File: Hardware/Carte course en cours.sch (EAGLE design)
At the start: 39 parts, among them J2 AVR_SPI_PROG_3X2NS, J3 PWR IN, J4 RC receiver, J5 ESC, J6 ESC, J7 MICRO-SD_CARD_SOCKET, J8 ESC, U1 V_REG_317SMD, U2 ATMEGA328P_TQFP, U3 FT232RL, U4 MPU6050, Y1 16MHz

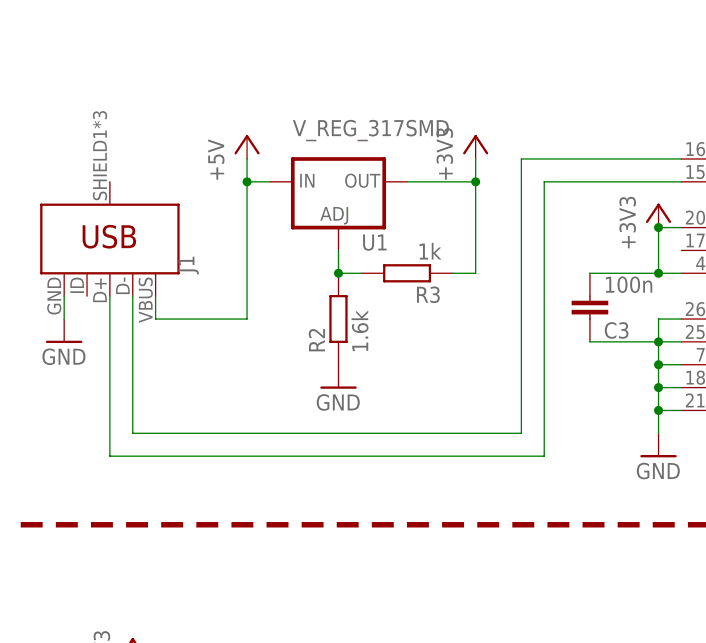
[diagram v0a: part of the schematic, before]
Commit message: Route
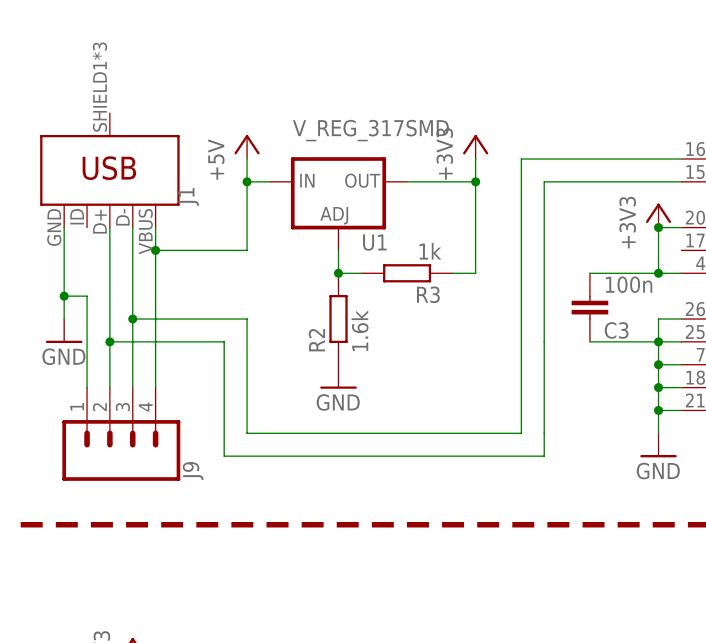
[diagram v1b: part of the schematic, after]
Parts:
- added J9: (no value), SparkFun-Connectors:CONN_04
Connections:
- net +5V: now also J9.4
- net GND: now also J9.1
- net N$2: now also J9.3
- net N$7: now also J9.2
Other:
- moved on the sheet: J1
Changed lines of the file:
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@@
 <setting verticaltext="up"/>
 </settings>
-<grid distance="0.1" unitdist="inch" unit="inch" style="lines" multiple="1" display="no" altdistance="0.01" altunitdist="inch" altunit="mil"/>
+<grid distance="0.1" unitdist="inch" unit="inch" style="lines" multiple="1" display="no" altdistance="0.01" altunitdist="inch" altunit="inch"/>
 <layers>
 <layer number="1" name="Top" color="4" fill="1" visible="no" active="no"/>
@@
 <part name="J5" library="SparkFun-Connectors" library_urn="urn:adsk.eagle:library:513" deviceset="CONN_02" device="" package3d_urn="urn:adsk.eagle:package:38039/1" value="ESC"/>
 <part name="J8" library="SparkFun-Connectors" library_urn="urn:adsk.eagle:library:513" deviceset="CONN_02" device="" package3d_urn="urn:adsk.eagle:package:38039/1" value="ESC"/>
+<part name="J9" library="SparkFun-Connectors" library_urn="urn:adsk.eagle:library:513" deviceset="CONN_04" device="" package3d_urn="urn:adsk.eagle:package:38085/1"/>
 </parts>
 <sheets>
@@
 <instance part="GND7" gate="1" x="83.82" y="106.68"/>
 <instance part="U3" gate="G$1" x="88.9" y="160.02"/>
-<instance part="J1" gate="G$1" x="10.16" y="162.56" rot="MR90"/>
+<instance part="J1" gate="G$1" x="10.16" y="170.18" rot="MR90"/>
 <instance part="GND1" gate="1" x="5.08" y="152.4"/>
 <instance part="C3" gate="G$1" x="63.5" y="154.94" rot="MR180"/>
@@
 <instance part="J5" gate="G$1" x="154.94" y="96.52" rot="MR0"/>
 <instance part="J8" gate="G$1" x="154.94" y="104.14" rot="MR0"/>
+<instance part="J9" gate="G$1" x="10.16" y="142.24" rot="MR90"/>
 </instances>
 <busses>
@@
 <pinref part="GND1" gate="1" pin="GND"/>
 <wire x1="5.08" y1="154.94" x2="5.08" y2="157.48" width="0.1524" layer="91"/>
+<pinref part="J9" gate="G$1" pin="1"/>
+<wire x1="5.08" y1="157.48" x2="5.08" y2="165.1" width="0.1524" layer="91"/>
+<wire x1="5.08" y1="157.48" x2="7.62" y2="157.48" width="0.1524" layer="91"/>
+<wire x1="7.62" y1="157.48" x2="7.62" y2="147.32" width="0.1524" layer="91"/>
+<junction x="5.08" y="157.48"/>
 </segment>
 <segment>
@@
 <segment>
 <pinref part="J1" gate="G$1" pin="VBUS"/>
-<wire x1="15.24" y1="157.48" x2="15.24" y2="154.94" width="0.1524" layer="91"/>
-<wire x1="15.24" y1="154.94" x2="25.4" y2="154.94" width="0.1524" layer="91"/>
-<wire x1="25.4" y1="154.94" x2="25.4" y2="170.18" width="0.1524" layer="91"/>
+<wire x1="15.24" y1="165.1" x2="15.24" y2="162.56" width="0.1524" layer="91"/>
+<wire x1="15.24" y1="162.56" x2="25.4" y2="162.56" width="0.1524" layer="91"/>
+<wire x1="25.4" y1="162.56" x2="25.4" y2="170.18" width="0.1524" layer="91"/>
 <pinref part="P+1" gate="1" pin="+5V"/>
 <pinref part="U1" gate="G$1" pin="IN"/>
@@
 <wire x1="27.94" y1="170.18" x2="25.4" y2="170.18" width="0.1524" layer="91"/>
 <junction x="25.4" y="170.18"/>
+<pinref part="J9" gate="G$1" pin="4"/>
+<wire x1="15.24" y1="162.56" x2="15.24" y2="147.32" width="0.1524" layer="91"/>
+<junction x="15.24" y="162.56"/>
 </segment>
 </net>
@@
 <segment>
 <pinref part="J1" gate="G$1" pin="D-"/>
-<wire x1="12.7" y1="157.48" x2="12.7" y2="142.24" width="0.1524" layer="91"/>
-<wire x1="12.7" y1="142.24" x2="55.88" y2="142.24" width="0.1524" layer="91"/>
+<wire x1="12.7" y1="165.1" x2="12.7" y2="154.94" width="0.1524" layer="91"/>
+<wire x1="12.7" y1="154.94" x2="25.4" y2="154.94" width="0.1524" layer="91"/>
+<wire x1="25.4" y1="154.94" x2="25.4" y2="142.24" width="0.1524" layer="91"/>
+<wire x1="25.4" y1="142.24" x2="55.88" y2="142.24" width="0.1524" layer="91"/>
 <wire x1="55.88" y1="142.24" x2="55.88" y2="172.72" width="0.1524" layer="91"/>
 <wire x1="55.88" y1="172.72" x2="73.66" y2="172.72" width="0.1524" layer="91"/>
 <pinref part="U3" gate="G$1" pin="USBDM"/>
+<pinref part="J9" gate="G$1" pin="3"/>
+<wire x1="12.7" y1="154.94" x2="12.7" y2="147.32" width="0.1524" layer="91"/>
+<junction x="12.7" y="154.94"/>
 </segment>
 </net>
@@
 <pinref part="J1" gate="G$1" pin="D+"/>
 <pinref part="U3" gate="G$1" pin="USBDP"/>
-<wire x1="10.16" y1="157.48" x2="10.16" y2="139.7" width="0.1524" layer="91"/>
-<wire x1="10.16" y1="139.7" x2="58.42" y2="139.7" width="0.1524" layer="91"/>
-<wire x1="58.42" y1="139.7" x2="58.42" y2="170.18" width="0.1524" layer="91"/>
+<wire x1="10.16" y1="165.1" x2="10.16" y2="152.4" width="0.1524" layer="91"/>
+<wire x1="10.16" y1="152.4" x2="22.86" y2="152.4" width="0.1524" layer="91"/>
+<wire x1="22.86" y1="152.4" x2="22.86" y2="139.7" width="0.1524" layer="91"/>
+<wire x1="22.86" y1="139.7" x2="58.42" y2="139.7" width="0.1524" layer="91"/>
+<wire x1="58.42" y1="139.7" x2="58.42" y2="142.24" width="0.1524" layer="91"/>
+<wire x1="58.42" y1="142.24" x2="58.42" y2="152.4" width="0.1524" layer="91"/>
+<wire x1="58.42" y1="152.4" x2="58.42" y2="170.18" width="0.1524" layer="91"/>
 <wire x1="58.42" y1="170.18" x2="73.66" y2="170.18" width="0.1524" layer="91"/>
-</segment>
-</net>
+<pinref part="J9" gate="G$1" pin="2"/>
+<wire x1="10.16" y1="152.4" x2="10.16" y2="147.32" width="0.1524" layer="91"/>
+<junction x="10.16" y="152.4"/>
+</segment>
+</net>
